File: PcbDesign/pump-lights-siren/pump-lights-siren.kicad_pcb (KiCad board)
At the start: 4 copper layers, 69.3 x 53.8 mm, 41 parts, among them J1 Conn_01x02_Socket, J2 Conn_01x02_Socket, J3 Conn_01x02_Socket, J4 Conn_01x02_Socket, Q1 Q_NMOS_GDS, Q2 Q_NMOS_GDS, Q3 Q_NMOS_GDS

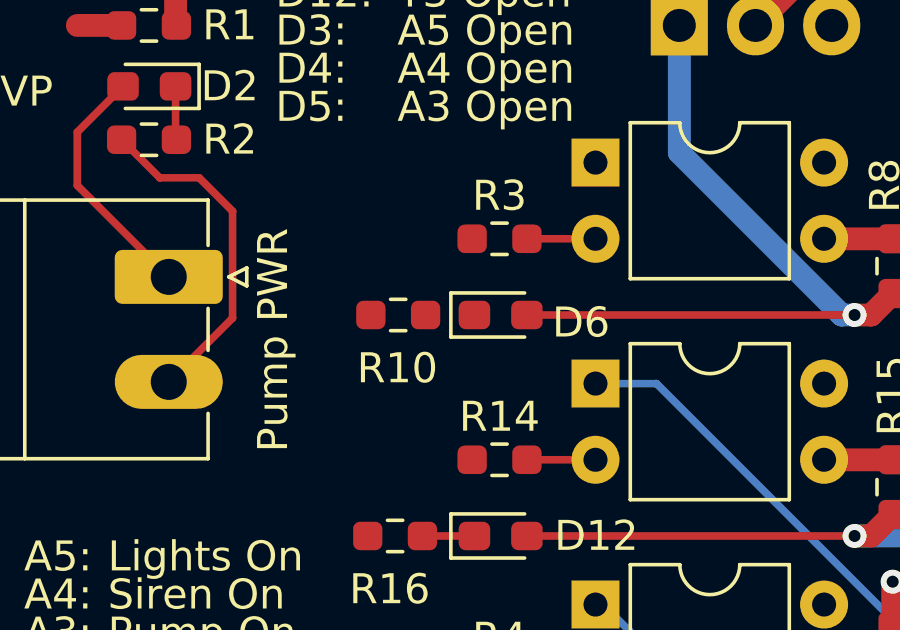
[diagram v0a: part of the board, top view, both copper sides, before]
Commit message: Routing Error
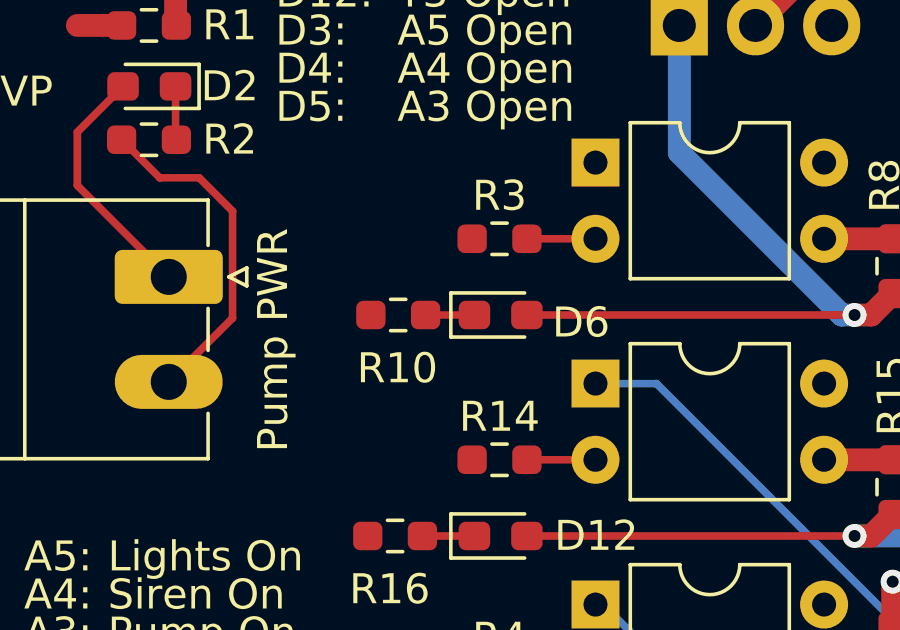
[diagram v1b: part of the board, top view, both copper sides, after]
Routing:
- net Net-(D6-K): track 0.00 -> 1.63 mm
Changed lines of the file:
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@@
   (segment (start 135.128 105.918) (end 147.165 93.881) (width 0.762) (layer "F.Cu") (net 57))
   (segment (start 160.119 93.881) (end 165.1 88.9) (width 0.762) (layer "F.Cu") (net 57))
+  (segment (start 125.758 115.57) (end 124.1305 115.57) (width 0.25) (layer "F.Cu") (net 58))
   (segment (start 130.048 130.81) (end 128.016 130.81) (width 0.254) (layer "F.Cu") (net 59))
   (segment (start 125.758 122.936) (end 124.027 122.936) (width 0.254) (layer "F.Cu") (net 60))
